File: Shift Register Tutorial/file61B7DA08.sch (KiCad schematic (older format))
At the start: 2 parts, among them SW401 SW_Push

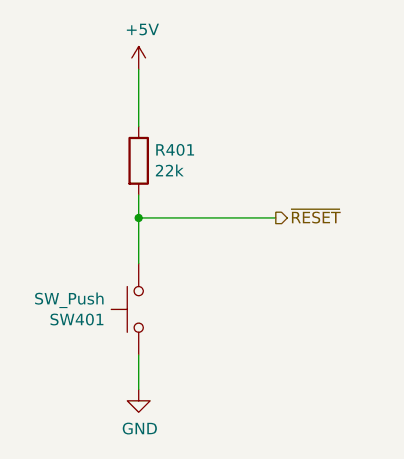
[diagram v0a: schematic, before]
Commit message: Working circuit together
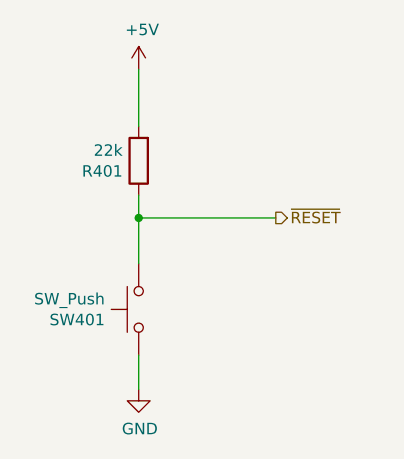
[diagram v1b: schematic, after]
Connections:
- net +5V: now also R401.2; no longer R401.1
- net ~RESET: now also R401.1; no longer R401.2
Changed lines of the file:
@@
 F 3 "~" H 2500 2300 50  0001 C CNN
 	1    2500 2300
-	1    0    0    -1
+	-1   0    0    1
 $EndComp
 $Comp
